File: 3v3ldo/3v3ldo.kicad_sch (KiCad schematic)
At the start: 3 parts

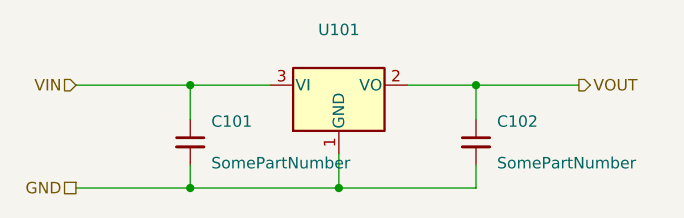
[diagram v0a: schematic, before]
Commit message: Reapply "Update modules to kicad v7 format"
This reverts commit fa5cc85431189ac7a3beedf0871b5723203ae43f.
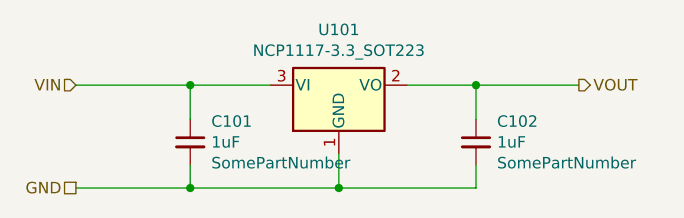
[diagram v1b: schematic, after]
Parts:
- C101, C102: value (none) -> 1uF; footprint (none) -> Capacitor_SMD:C_0603_1608Metric
- U101: value (none) -> NCP1117-3.3_SOT223; footprint (none) -> Package_TO_SOT_SMD:SOT-223-3_TabPin2
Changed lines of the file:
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@@
-(kicad_sch (version 20211123) (generator eeschema)
+(kicad_sch (version 20230121) (generator eeschema)
   (paper "A4")
   (title_block
@@
   )
   (wire (pts (xy 161.29 93.98) (xy 161.29 90.17))
-    (stroke (width 0) (type default) (color 0 0 0 0))
+    (stroke (width 0) (type default))
   )
   (wire (pts (xy 129.54 101.6) (xy 146.05 101.6))
-    (stroke (width 0) (type default) (color 0 0 0 0))
+    (stroke (width 0) (type default))
   )
   (wire (pts (xy 129.54 101.6) (xy 116.84 101.6))
-    (stroke (width 0) (type default) (color 0 0 0 0))
+    (stroke (width 0) (type default))
   )
   (wire (pts (xy 138.43 90.17) (xy 129.54 90.17))
-    (stroke (width 0) (type default) (color 0 0 0 0))
+    (stroke (width 0) (type default))
   )
   (wire (pts (xy 129.54 90.17) (xy 116.84 90.17))
-    (stroke (width 0) (type default) (color 0 0 0 0))
+    (stroke (width 0) (type default))
   )
   (wire (pts (xy 161.29 90.17) (xy 172.72 90.17))
-    (stroke (width 0) (type default) (color 0 0 0 0))
+    (stroke (width 0) (type default))
   )
   (wire (pts (xy 129.54 99.06) (xy 129.54 101.6))
-    (stroke (width 0) (type default) (color 0 0 0 0))
+    (stroke (width 0) (type default))
   )
   (wire (pts (xy 146.05 101.6) (xy 161.29 101.6))
-    (stroke (width 0) (type default) (color 0 0 0 0))
+    (stroke (width 0) (type default))
   )
   (wire (pts (xy 129.54 90.17) (xy 129.54 93.98))
-    (stroke (width 0) (type default) (color 0 0 0 0))
+    (stroke (width 0) (type default))
   )
   (wire (pts (xy 161.29 101.6) (xy 161.29 99.06))
-    (stroke (width 0) (type default) (color 0 0 0 0))
+    (stroke (width 0) (type default))
   )
   (wire (pts (xy 146.05 97.79) (xy 146.05 101.6))
-    (stroke (width 0) (type default) (color 0 0 0 0))
+    (stroke (width 0) (type default))
   )
   (wire (pts (xy 161.29 90.17) (xy 153.67 90.17))
-    (stroke (width 0) (type default) (color 0 0 0 0))
+    (stroke (width 0) (type default))
   )
-  (hierarchical_label "GND" (shape passive) (at 116.84 101.6 180)
+  (hierarchical_label "GND" (shape passive) (at 116.84 101.6 180) (fields_autoplaced)
     (effects (font (size 1.27 1.27)) (justify right))
   )
-  (hierarchical_label "VOUT" (shape output) (at 172.72 90.17 0)
+  (hierarchical_label "VOUT" (shape output) (at 172.72 90.17 0) (fields_autoplaced)
     (effects (font (size 1.27 1.27)) (justify left))
   )
-  (hierarchical_label "VIN" (shape input) (at 116.84 90.17 180)
+  (hierarchical_label "VIN" (shape input) (at 116.84 90.17 180) (fields_autoplaced)
     (effects (font (size 1.27 1.27)) (justify right))
   )
   (symbol (lib_id "Regulator_Linear:NCP1117-3.3_SOT223") (at 146.05 90.17 0) (unit 1)
-    (in_bom yes) (on_board yes)
-    (property "Reference" "U101" (id 0) (at 146.05 84.0232 0))
-    (property "Value" "" (id 1) (at 146.05 86.3346 0))
-    (property "Footprint" "" (id 2) (at 146.05 85.09 0)
+    (in_bom yes) (on_board yes) (dnp no)
+    (property "Reference" "U101" (at 146.05 84.0232 0)
+      (effects (font (size 1.27 1.27)))
+    )
+    (property "Value" "NCP1117-3.3_SOT223" (at 146.05 86.3346 0)
+      (effects (font (size 1.27 1.27)))
+    )
+    (property "Footprint" "Package_TO_SOT_SMD:SOT-223-3_TabPin2" (at 146.05 85.09 0)
       (effects (font (size 1.27 1.27)) hide)
     )
-    (property "Datasheet" "http://www.onsemi.com/pub_link/Collateral/NCP1117-D.PDF" (id 3) (at 148.59 96.52 0)
+    (property "Datasheet" "http://www.onsemi.com/pub_link/Collateral/NCP1117-D.PDF" (at 148.59 96.52 0)
       (effects (font (size 1.27 1.27)) hide)
     )
@@
     (pin "2")
     (pin "3")
+    (instances
+      (project "3v3ldo"
+        (path "/554e6850-3780-446a-9126-30efe96707a4"
+          (reference "U101") (unit 1)
+        )
+      )
+    )
   )
   (symbol (lib_id "Device:C_Small") (at 129.54 96.52 0) (unit 1)
-    (in_bom yes) (on_board yes)
-    (property "Reference" "C101" (id 0) (at 131.8768 94.2086 0)
+    (in_bom yes) (on_board yes) (dnp no)
+    (property "Reference" "C101" (at 131.8768 94.2086 0)
       (effects (font (size 1.27 1.27)) (justify left))
     )
-    (property "Value" "" (id 1) (at 131.8768 96.52 0)
+    (property "Value" "1uF" (at 131.8768 96.52 0)
       (effects (font (size 1.27 1.27)) (justify left))
     )
-    (property "Footprint" "" (id 2) (at 129.54 96.52 0)
+    (property "Footprint" "Capacitor_SMD:C_0603_1608Metric" (at 129.54 96.52 0)
       (effects (font (size 1.27 1.27)) hide)
     )
-    (property "Datasheet" "~" (id 3) (at 129.54 96.52 0)
+    (property "Datasheet" "~" (at 129.54 96.52 0)
       (effects (font (size 1.27 1.27)) hide)
     )
-    (property "PartNo" "SomePartNumber" (id 4) (at 131.8768 98.8314 0)
+    (property "PartNo" "SomePartNumber" (at 131.8768 98.8314 0)
       (effects (font (size 1.27 1.27)) (justify left))
     )
     (pin "1")
     (pin "2")
+    (instances
+      (project "3v3ldo"
+        (path "/554e6850-3780-446a-9126-30efe96707a4"
+          (reference "C101") (unit 1)
+        )
+      )
+    )
   )
   (symbol (lib_id "Device:C_Small") (at 161.29 96.52 0) (unit 1)
-    (in_bom yes) (on_board yes)
-    (property "Reference" "C102" (id 0) (at 163.6268 94.2086 0)
+    (in_bom yes) (on_board yes) (dnp no)
+    (property "Reference" "C102" (at 163.6268 94.2086 0)
       (effects (font (size 1.27 1.27)) (justify left))
     )
-    (property "Value" "" (id 1) (at 163.6268 96.52 0)
+    (property "Value" "1uF" (at 163.6268 96.52 0)
       (effects (font (size 1.27 1.27)) (justify left))
     )
-    (property "Footprint" "" (id 2) (at 161.29 96.52 0)
+    (property "Footprint" "Capacitor_SMD:C_0603_1608Metric" (at 161.29 96.52 0)
       (effects (font (size 1.27 1.27)) hide)
     )
-    (property "Datasheet" "~" (id 3) (at 161.29 96.52 0)
+    (property "Datasheet" "~" (at 161.29 96.52 0)
       (effects (font (size 1.27 1.27)) hide)
     )
-    (property "PartNo" "SomePartNumber" (id 4) (at 163.6268 98.8314 0)
+    (property "PartNo" "SomePartNumber" (at 163.6268 98.8314 0)
       (effects (font (size 1.27 1.27)) (justify left))
     )
     (pin "1")
     (pin "2")
+    (instances
+      (project "3v3ldo"
+        (path "/554e6850-3780-446a-9126-30efe96707a4"
+          (reference "C102") (unit 1)
+        )
+      )
+    )
   )
   (sheet_instances
     (path "/" (page "1"))
   )
-  (symbol_instances
-    (path "/00000000-0000-0000-0000-00005e248390"
-      (reference "C101") (unit 1) (value "1uF") (footprint "Capacitor_SMD:C_0603_1608Metric")
-    )
-    (path "/00000000-0000-0000-0000-00005e24895c"
-      (reference "C102") (unit 1) (value "1uF") (footprint "Capacitor_SMD:C_0603_1608Metric")
-    )
-    (path "/00000000-0000-0000-0000-00005e246b49"
-      (reference "U101") (unit 1) (value "NCP1117-3.3_SOT223") (footprint "Package_TO_SOT_SMD:SOT-223-3_TabPin2")
-    )
-  )
 )
